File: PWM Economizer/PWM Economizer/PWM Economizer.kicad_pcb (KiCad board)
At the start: 2 copper layers, 68 x 52 mm, 99 parts, among them J1 Conn_01x08_Pin, Q1 PNP, Q2 PNP, U1 DRV103 SO-8, U2 TPS7B8250QDGNRQ1, U3 DRV103 SO-8

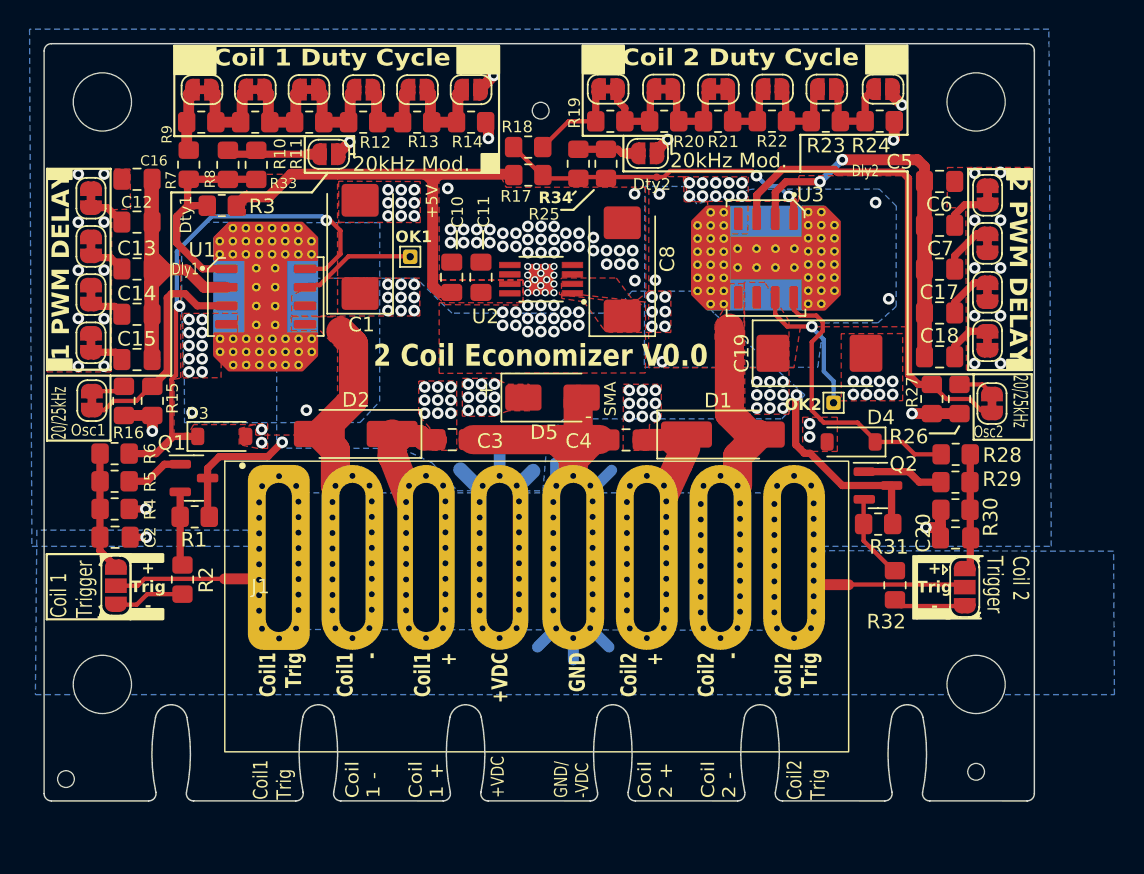
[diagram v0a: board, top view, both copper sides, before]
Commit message: V1.1 Untested
V1.1 Untested
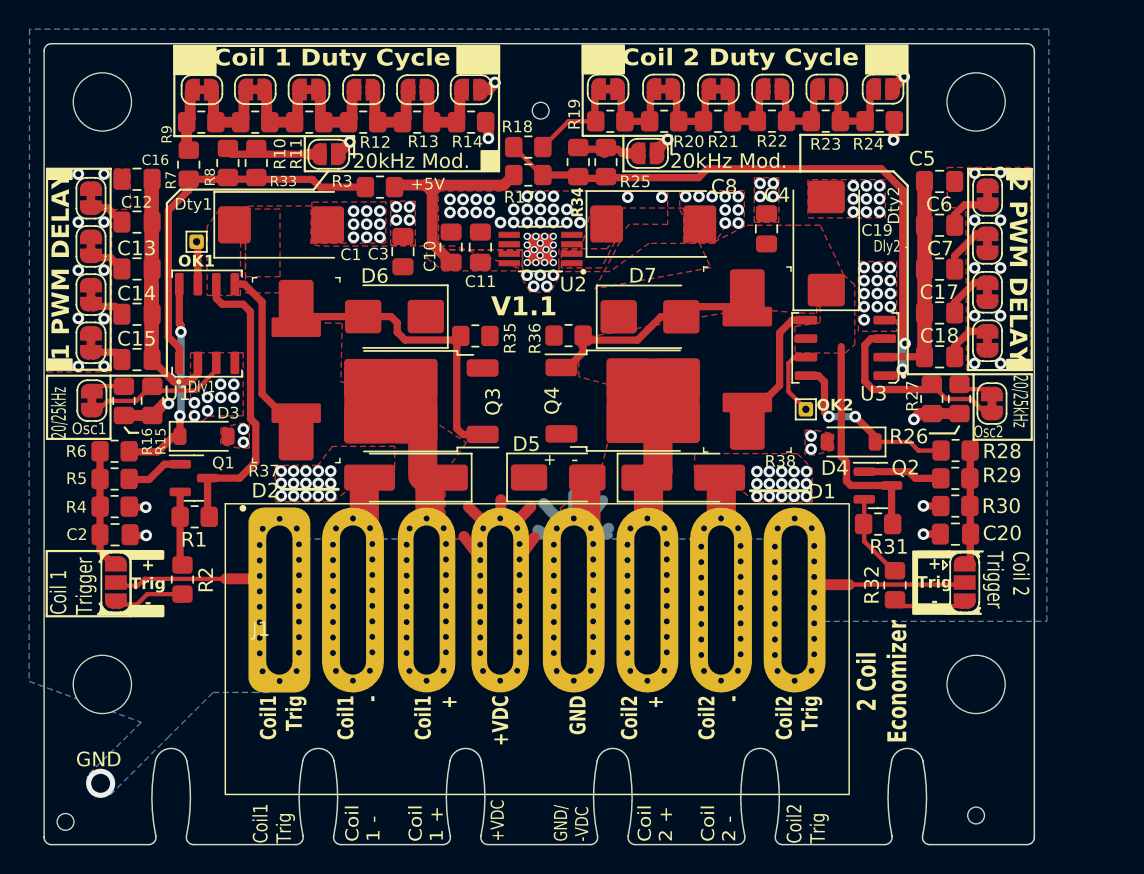
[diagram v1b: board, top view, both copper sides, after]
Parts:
- added D6: D_16V_Zener, Diode_SMD:D_SMB, F.Cu at (70.1, 74.7)
- added D7: D_16V_Zener, Diode_SMD:D_SMB, F.Cu at (87.6, 74.8)
- added G***: LOGO, 2 Coil Economizer Github Link:2 Coil Economizer Github Link, B.Cu at (79.9, 77.0)
- added Q3: SUD50P10-43L, Package_TO_SOT_SMD:TO-252-2, F.Cu at (71.1, 80.5)
- added Q4: SUD50P10-43L, Package_TO_SOT_SMD:TO-252-2, F.Cu at (86.6, 80.5)
- added R35: 3k, Resistor_SMD:R_0805_2012Metric_Pad1.20x1.40mm_HandSolder, F.Cu at (75.6, 76.1)
- added R36: 3k, Resistor_SMD:R_0805_2012Metric_Pad1.20x1.40mm_HandSolder, F.Cu at (82.0, 76.0)
- added R37: 100R 2W/3W, SMD_Res_footprints:SMD_Res 3W 12x5.8 & 2512, F.Cu at (63.3, 78.4)
- added R38: 100R 2W/3W, SMD_Res_footprints:SMD_Res 3W 12x5.8 & 2512, F.Cu at (94.3, 77.7)
- U1, U3: footprint DRV103:DRV103 PowerPad SOIC Large Heatsink -> DRV103:DRV103 No Heatsink
- moved C4 17.4 mm to (95.6, 68.7), turned to 90 degrees
- moved TP1 14.7 mm to (56.5, 69.6), turned to -90 degrees
- moved C3 13.3 mm to (70.6, 70.3), turned to 90 degrees
- moved R3 10.9 mm to (69.1, 65.8)
- moved U3 8.23 mm to (101.0, 76.9), turned to 180 degrees
- moved C19 7.55 mm to (99.7, 69.7), turned to 90 degrees
- moved C1 5.64 mm to (62.3, 68.4), turned to 0 degrees
- moved D5 5.50 mm to (81.3, 85.8)
- moved D2 4.57 mm to (70.8, 85.8)
- moved U1 4.44 mm to (57.2, 75.2), turned to 90 degrees
- moved D1 4.02 mm to (89.9, 85.8)
- moved C8 3.78 mm to (87.8, 68.4), turned to 0 degrees
- moved REF** 3.00 mm to (110.0, 109.0)
- moved REF** 2.94 mm to (47.5, 109.4)
- moved J1 2.93 mm to (79.9, 96.7)
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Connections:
- C1 pad 1: Coil1+ -> +VDC
- C19 pad 1: Coil1+ -> +VDC
- C3 pad 1: Coil1+ -> +VDC
- C4 pad 1: Coil1+ -> +VDC
- C8 pad 1: Coil1+ -> +VDC
- D1 pad 1: Coil1+ -> Coil2+
- D1 pad 2: Coil2- -> GND
- D2 pad 2: Coil1- -> GND
- D5 pad 1: Coil1+ -> +VDC
- J1 pad 2: Coil1- -> GND
- J1 pad 4: Coil1+ -> +VDC
- J1 pad 6: Coil1+ -> Coil2+
- J1 pad 7: Coil2- -> GND
- Q1 pad 3: Coil1+ -> +VDC
- Q2 pad 3: Coil1+ -> +VDC
- R1 pad 1: Coil1+ -> +VDC
- R31 pad 1: Coil1+ -> +VDC
- U1 pad 5: Coil1- -> Net-(U1-OUT)
- U1 pad 6: Coil1+ -> +VDC
- U2 pad 1: Coil1+ -> +VDC
- U2 pad 2: Coil1+ -> +VDC
- U3 pad 5: Coil2- -> Net-(U3-OUT)
- U3 pad 6: Coil1+ -> +VDC
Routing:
- net +VDC: track 0.00 -> 52.4 mm
- net Coil1+: track 49.8 -> 12.6 mm, vias 53 -> 0
- net Input1: track 35.4 -> 14.4 mm
- net Net-(D6-A): track 0.00 -> 20.5 mm
- net DutyCycAdj2: track 22.8 -> 43.0 mm
- net OSC_Adj2: track 33.3 -> 14.0 mm
- net Coil1-: track 16.4 -> 0.00 mm
- net +5V: track 31.1 -> 15.4 mm
- net Net-(D7-A): track 0.00 -> 14.3 mm
- net Coil2+: track 0.00 -> 13.1 mm
- net Net-(U1-OUT): track 0.00 -> 12.8 mm
- net Coil2-: track 12.6 -> 0.00 mm
- net Delay_Adj2: track 27.7 -> 16.2 mm, vias 2 -> 0
- net DutyCycAdj1: track 14.9 -> 26.1 mm
- net Net-(U3-OUT): track 0.00 -> 9.63 mm
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- added copper zone on F.Cu, net +VDC
- removed copper zone on B.Cu, net Coil1+
- removed copper zone on F.Cu, net Coil1+
- removed copper zone on F.Cu, net Coil1-
- removed copper zone on F.Cu, net Coil2-
- removed copper zone on B.Cu, net HS1
- removed copper zone on F.Cu, net HS1
- removed copper zone on B.Cu, net HS2
- removed copper zone on F.Cu, net HS2
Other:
- board size 68 x 52 mm -> 68 x 55 mm
- board text added: "2 Coil Economizer"
- board text added: "Dly2 -"
- board text added: "GND"
- board text added: "Must feed + & - to coils through their connections on this board. +VDC is +12V. Designed to work from 8v - ~28vdc."
- board text added: "V1.1"
- board text removed: "2 Coil Economizer V0.0"
- board text removed: "Dly2"
- board text removed: "Must feed + to coils thru their connections on this board. +VDC is +12V. Designed to work from 8v - ~28vdc. D5 is an SMA footprint for a TVS diode."
- board text removed: "SMA"
